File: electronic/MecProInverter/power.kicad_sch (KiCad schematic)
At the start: 87 parts, among them J10 Net, J4 Motor, J8 U_ZK, J9 U_VS, K2 RT314A12, Q1 DMN3404L, U10 CC6904SO-30A, U11 CC6904SO-30A, U13 IKCM20L60GA, U4 LVE2560E, U5 TPS563201DDCR, U8 TLA2528IRTER, U9 CC6904SO-30A

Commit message: Electronic
Voltage messurment updated
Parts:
- added C53, C54, C55: C, symbol Device:C
- added R63, R64: 33k, Resistor_SMD:R_1206_3216Metric, symbol Device:R
- R41: value 10k -> 4,7k
- R46: value 100k -> 33k; footprint Resistor_SMD:R_0201_0603Metric_Pad0.64x0.40mm_HandSolder -> Resistor_SMD:R_1206_3216Metric
- R60: value 999m -> 330; footprint Resistor_SMD:R_0201_0603Metric_Pad0.64x0.40mm_HandSolder -> (none)
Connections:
- net GND: now also C53.2, C54.2, C55.2; no longer R60.2
- net ITRIP: no longer C51.1, R41.2, U13.15 (ITRIP)
- net at R47.1, U8.1 (AIN2/GPIO2): now also C55.1, R64.2; no longer R46.2
- net at R33.1, R34.2, U8.15 (AIN0/GPIO0): now also C54.1
- net at R61.2, R62.1, U8.16 (AIN1/GPIO1): now also C53.1
- net at U9.1 (IP+), U9.2 (IP+): now also U4.1 (VDD); no longer K2.14, R1.2
- net at U9.3 (IP-), U9.4 (IP-): now also C1.1, C2.1, C3.1, C4.1, J8.1 (Pin_1), U13.23 (P), R63.1; no longer U4.2 (~Phase)
- new net: K2.14, R1.2, U4.2 (~Phase)
- new net: R46.1, R63.2
- new net: R46.2, R64.1
- new net: C51.1, R41.2, R60.2, U13.15 (ITRIP)
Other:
- moved on the sheet: C1, C10, C11, C12, C13, C14, C15, C16, C17, C18, C19, C2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

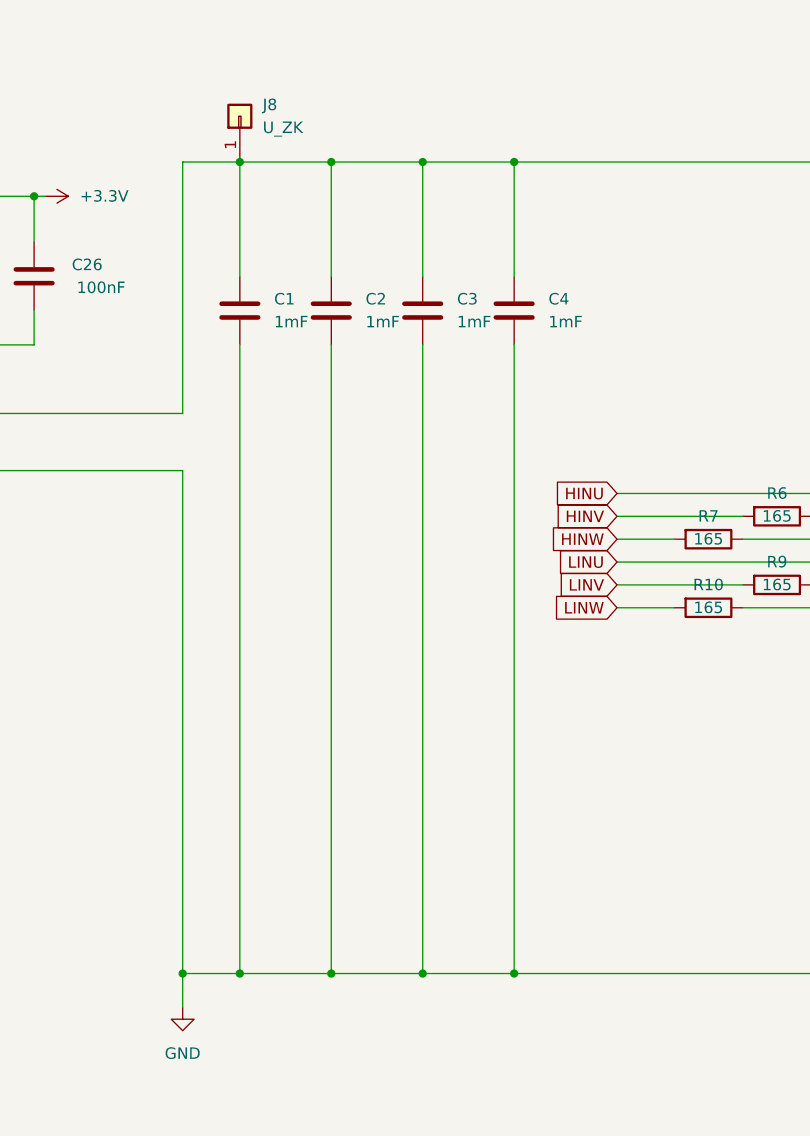
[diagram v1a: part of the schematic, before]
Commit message: Electronic
docu
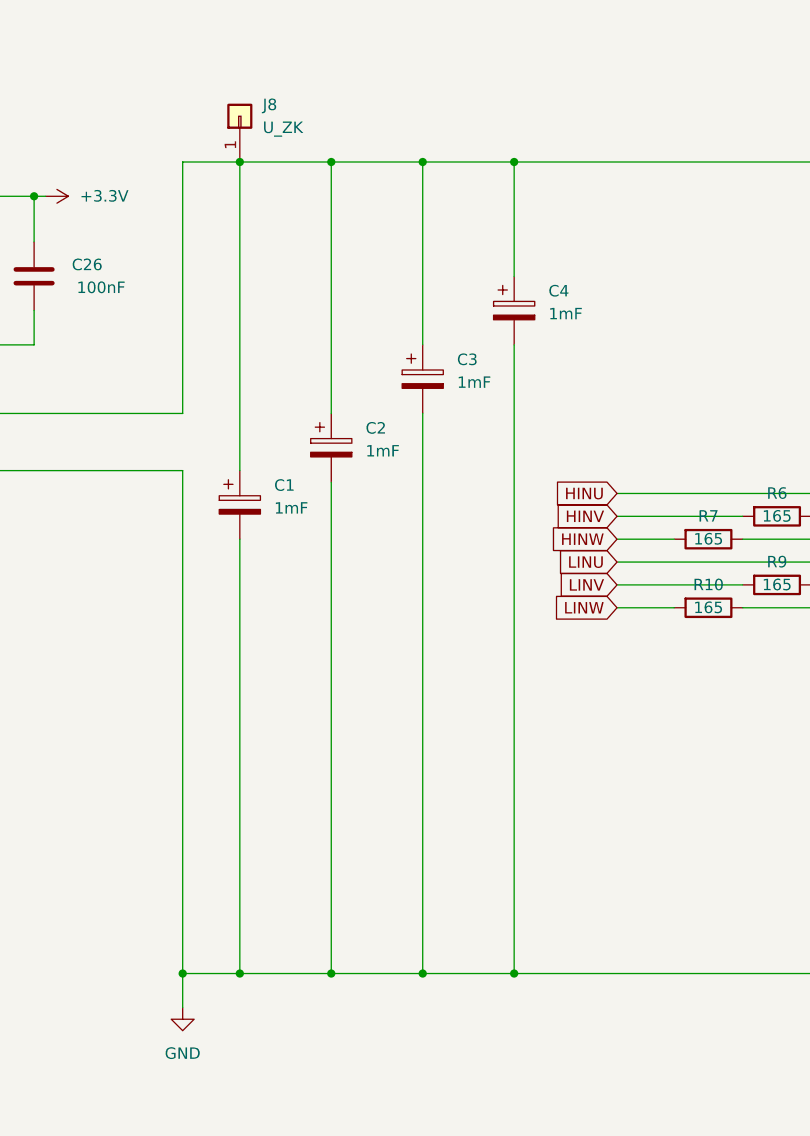
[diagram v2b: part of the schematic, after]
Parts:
- removed C1, C2, C3, C4: 1mF, footprints:ESMQ351VSN102MA50S, symbol Device:C
- added C1, C2, C3, C4: 1mF, Own_Footprint:ESMQ351VSN102MA50S, symbol Device:C_Polarized
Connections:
- net GND: now also C1.2, C2.2, C3.2, C4.2
- net at J8.1 (Pin_1), R63.1, U13.23 (P)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: now also C1.1, C2.1, C3.1, C4.1
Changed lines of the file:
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@@
     (stroke (width 0) (type default))
   )
-  (wire (pts (xy 222.25 127) (xy 222.25 196.85))
+  (wire (pts (xy 222.25 142.24) (xy 222.25 196.85))
     (stroke (width 0) (type default))
   )
@@
     (stroke (width 0) (type default))
   )
-  (wire (pts (xy 232.41 127) (xy 232.41 196.85))
+  (wire (pts (xy 232.41 134.62) (xy 232.41 196.85))
     (stroke (width 0) (type default))
   )
@@
     (stroke (width 0) (type default))
   )
-  (wire (pts (xy 212.09 106.68) (xy 212.09 119.38))
+  (wire (pts (xy 212.09 106.68) (xy 212.09 140.97))
     (stroke (width 0) (type default))
   )
@@
     (stroke (width 0) (type default))
   )
-  (wire (pts (xy 222.25 106.68) (xy 222.25 119.38))
+  (wire (pts (xy 222.25 106.68) (xy 222.25 134.62))
     (stroke (width 0) (type default))
   )
@@
     (stroke (width 0) (type default))
   )
-  (wire (pts (xy 232.41 106.68) (xy 232.41 119.38))
+  (wire (pts (xy 232.41 106.68) (xy 232.41 127))
     (stroke (width 0) (type default))
   )
@@
     (stroke (width 0) (type default))
   )
-  (wire (pts (xy 212.09 127) (xy 212.09 196.85))
+  (wire (pts (xy 212.09 148.59) (xy 212.09 196.85))
     (stroke (width 0) (type default))
   )
@@
     )
   )
-  (symbol (lib_id "Device:C") (at 222.25 123.19 0) (unit 1)
-    (in_bom yes) (on_board yes) (dnp no) (fields_autoplaced)
-    (property "Reference" "C2" (at 226.06 121.92 0)
-      (effects (font (size 1.27 1.27)) (justify left))
-    )
-    (property "Value" "1mF" (at 226.06 124.46 0)
-      (effects (font (size 1.27 1.27)) (justify left))
-    )
-    (property "Footprint" "footprints:ESMQ351VSN102MA50S" (at 223.2152 127 0)
-      (effects (font (size 1.27 1.27)) hide)
-    )
-    (property "Datasheet" "~" (at 222.25 123.19 0)
-      (effects (font (size 1.27 1.27)) hide)
-    )
-    (pin "1")
-    (pin "2")
-    (instances
-      (project "MecProInverter"
-        (path "/c9071429-8b0d-45bf-aa6d-71cc2b7f068c/c32f479b-361e-4c54-ac43-ed36ba4d4493"
-          (reference "C2") (unit 1)
-        )
-      )
-    )
-  )
   (symbol (lib_id "Device:R") (at 179.07 288.29 180) (unit 1)
     (in_bom yes) (on_board yes) (dnp no)
@@
     )
   )
+  (symbol (lib_id "Device:C_Polarized") (at 242.57 123.19 0) (unit 1)
+    (in_bom yes) (on_board yes) (dnp no) (fields_autoplaced)
+    (property "Reference" "C4" (at 246.38 121.031 0)
+      (effects (font (size 1.27 1.27)) (justify left))
+    )
+    (property "Value" "1mF" (at 246.38 123.571 0)
+      (effects (font (size 1.27 1.27)) (justify left))
+    )
+    (property "Footprint" "Own_Footprint:ESMQ351VSN102MA50S" (at 243.5352 127 0)
+      (effects (font (size 1.27 1.27)) hide)
+    )
+    (property "Datasheet" "~" (at 242.57 123.19 0)
+      (effects (font (size 1.27 1.27)) hide)
+    )
+    (pin "1")
+    (pin "2")
+    (instances
+      (project "MecProInverter"
+        (path "/c9071429-8b0d-45bf-aa6d-71cc2b7f068c/c32f479b-361e-4c54-ac43-ed36ba4d4493"
+          (reference "C4") (unit 1)
+        )
+      )
+    )
+  )
   (symbol (lib_id "Device:R") (at 62.23 134.62 90) (unit 1)
     (in_bom yes) (on_board yes) (dnp no)
@@
     )
   )
+  (symbol (lib_id "Device:C_Polarized") (at 222.25 138.43 0) (unit 1)
+    (in_bom yes) (on_board yes) (dnp no) (fields_autoplaced)
+    (property "Reference" "C2" (at 226.06 136.271 0)
+      (effects (font (size 1.27 1.27)) (justify left))
+    )
+    (property "Value" "1mF" (at 226.06 138.811 0)
+      (effects (font (size 1.27 1.27)) (justify left))
+    )
+    (property "Footprint" "Own_Footprint:ESMQ351VSN102MA50S" (at 223.2152 142.24 0)
+      (effects (font (size 1.27 1.27)) hide)
+    )
+    (property "Datasheet" "~" (at 222.25 138.43 0)
+      (effects (font (size 1.27 1.27)) hide)
+    )
+    (pin "1")
+    (pin "2")
+    (instances
+      (project "MecProInverter"
+        (path "/c9071429-8b0d-45bf-aa6d-71cc2b7f068c/c32f479b-361e-4c54-ac43-ed36ba4d4493"
+          (reference "C2") (unit 1)
+        )
+      )
+    )
+  )
   (symbol (lib_id "IKCM20L60GA:IKCM20L60GA") (at 358.14 143.51 0) (unit 1)
     (in_bom yes) (on_board yes) (dnp no) (fields_autoplaced)
@@
     )
   )
-  (symbol (lib_id "Device:C") (at 232.41 123.19 0) (unit 1)
-    (in_bom yes) (on_board yes) (dnp no) (fields_autoplaced)
-    (property "Reference" "C3" (at 236.22 121.92 0)
-      (effects (font (size 1.27 1.27)) (justify left))
-    )
-    (property "Value" "1mF" (at 236.22 124.46 0)
-      (effects (font (size 1.27 1.27)) (justify left))
-    )
-    (property "Footprint" "footprints:ESMQ351VSN102MA50S" (at 233.3752 127 0)
-      (effects (font (size 1.27 1.27)) hide)
-    )
-    (property "Datasheet" "~" (at 232.41 123.19 0)
-      (effects (font (size 1.27 1.27)) hide)
-    )
-    (pin "1")
-    (pin "2")
-    (instances
-      (project "MecProInverter"
-        (path "/c9071429-8b0d-45bf-aa6d-71cc2b7f068c/c32f479b-361e-4c54-ac43-ed36ba4d4493"
-          (reference "C3") (unit 1)
-        )
-      )
-    )
-  )
   (symbol (lib_id "Device:R") (at 264.16 156.21 270) (unit 1)
     (in_bom yes) (on_board yes) (dnp no)
@@
     )
   )
+  (symbol (lib_id "Device:C_Polarized") (at 232.41 130.81 0) (unit 1)
+    (in_bom yes) (on_board yes) (dnp no) (fields_autoplaced)
+    (property "Reference" "C3" (at 236.22 128.651 0)
+      (effects (font (size 1.27 1.27)) (justify left))
+    )
+    (property "Value" "1mF" (at 236.22 131.191 0)
+      (effects (font (size 1.27 1.27)) (justify left))
+    )
+    (property "Footprint" "Own_Footprint:ESMQ351VSN102MA50S" (at 233.3752 134.62 0)
+      (effects (font (size 1.27 1.27)) hide)
+    )
+    (property "Datasheet" "~" (at 232.41 130.81 0)
+      (effects (font (size 1.27 1.27)) hide)
+    )
+    (pin "1")
+    (pin "2")
+    (instances
+      (project "MecProInverter"
+        (path "/c9071429-8b0d-45bf-aa6d-71cc2b7f068c/c32f479b-361e-4c54-ac43-ed36ba4d4493"
+          (reference "C3") (unit 1)
+        )
+      )
+    )
+  )
   (symbol (lib_id "power:+3.3V") (at 571.5 144.78 270) (unit 1)
     (in_bom yes) (on_board yes) (dnp no) (fields_autoplaced)
@@
     )
   )
-  (symbol (lib_id "Device:C") (at 212.09 123.19 0) (unit 1)
-    (in_bom yes) (on_board yes) (dnp no) (fields_autoplaced)
-    (property "Reference" "C1" (at 215.9 121.92 0)
-      (effects (font (size 1.27 1.27)) (justify left))
-    )
-    (property "Value" "1mF" (at 215.9 124.46 0)
-      (effects (font (size 1.27 1.27)) (justify left))
-    )
-    (property "Footprint" "footprints:ESMQ351VSN102MA50S" (at 213.0552 127 0)
-      (effects (font (size 1.27 1.27)) hide)
-    )
-    (property "Datasheet" "~" (at 212.09 123.19 0)
-      (effects (font (size 1.27 1.27)) hide)
-    )
-    (pin "1")
-    (pin "2")
-    (instances
-      (project "MecProInverter"
-        (path "/c9071429-8b0d-45bf-aa6d-71cc2b7f068c/c32f479b-361e-4c54-ac43-ed36ba4d4493"
-          (reference "C1") (unit 1)
-        )
-      )
-    )
-  )
   (symbol (lib_id "Device:C") (at 189.23 119.38 180) (unit 1)
     (in_bom yes) (on_board yes) (dnp no)
@@
     )
   )
+  (symbol (lib_id "Device:C_Polarized") (at 212.09 144.78 0) (unit 1)
+    (in_bom yes) (on_board yes) (dnp no) (fields_autoplaced)
+    (property "Reference" "C1" (at 215.9 142.621 0)
+      (effects (font (size 1.27 1.27)) (justify left))
+    )
+    (property "Value" "1mF" (at 215.9 145.161 0)
+      (effects (font (size 1.27 1.27)) (justify left))
+    )
+    (property "Footprint" "Own_Footprint:ESMQ351VSN102MA50S" (at 213.0552 148.59 0)
+      (effects (font (size 1.27 1.27)) hide)
+    )
+    (property "Datasheet" "~" (at 212.09 144.78 0)
+      (effects (font (size 1.27 1.27)) hide)
+    )
+    (pin "1")
+    (pin "2")
+    (instances
+      (project "MecProInverter"
+        (path "/c9071429-8b0d-45bf-aa6d-71cc2b7f068c/c32f479b-361e-4c54-ac43-ed36ba4d4493"
+          (reference "C1") (unit 1)
+        )
+      )
+    )
+  )
   (symbol (lib_id "Device:C_Polarized") (at 316.23 118.11 270) (unit 1)
     (in_bom yes) (on_board yes) (dnp no) (fields_autoplaced)
@@
         )
       )
-    )
-  )
-  (symbol (lib_id "Device:C") (at 242.57 123.19 0) (unit 1)
-    (in_bom yes) (on_board yes) (dnp no) (fields_autoplaced)
-    (property "Reference" "C4" (at 246.38 121.92 0)
-      (effects (font (size 1.27 1.27)) (justify left))
-    )
-    (property "Value" "1mF" (at 246.38 124.46 0)
-      (effects (font (size 1.27 1.27)) (justify left))
-    )
-    (property "Footprint" "footprints:ESMQ351VSN102MA50S" (at 243.5352 127 0)
-      (effects (font (size 1.27 1.27)) hide)
-    )
-    (property "Datasheet" "~" (at 242.57 123.19 0)
-      (effects (font (size 1.27 1.27)) hide)
-    )
-    (pin "1")
-    (pin "2")
-    (instances
-      (project "MecProInverter"
-        (path "/c9071429-8b0d-45bf-aa6d-71cc2b7f068c/c32f479b-361e-4c54-ac43-ed36ba4d4493"
-          (reference "C4") (unit 1)
-        )
-      )

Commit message: Electronic
Added 3d Moodel on Layout
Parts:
- U4: footprint Own_Library:LVE2560E -> Own_Footprint:LVE2560E
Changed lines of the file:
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@@
       (effects (font (size 1.27 1.27)))
     )
-    (property "Footprint" "Own_Library:LVE2560E" (at 80.01 149.86 0)
+    (property "Footprint" "Own_Footprint:LVE2560E" (at 80.01 149.86 0)
       (effects (font (size 1.27 1.27)) hide)
     )
